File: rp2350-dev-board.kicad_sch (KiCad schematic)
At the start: 49 parts, among them J1 USB4105-GF-A, J2 Conn_02x20_Odd_Even, J3 Conn_02x20_Odd_Even, SW1 RST, SW2 BOOTSEL, U1 W25Q128JVS, U2 RP2350B, U3 TPS6285021HQDRLRQ1, U4 LM66100DCK, Y1 ABM8-272-T3 12MHz/10pF

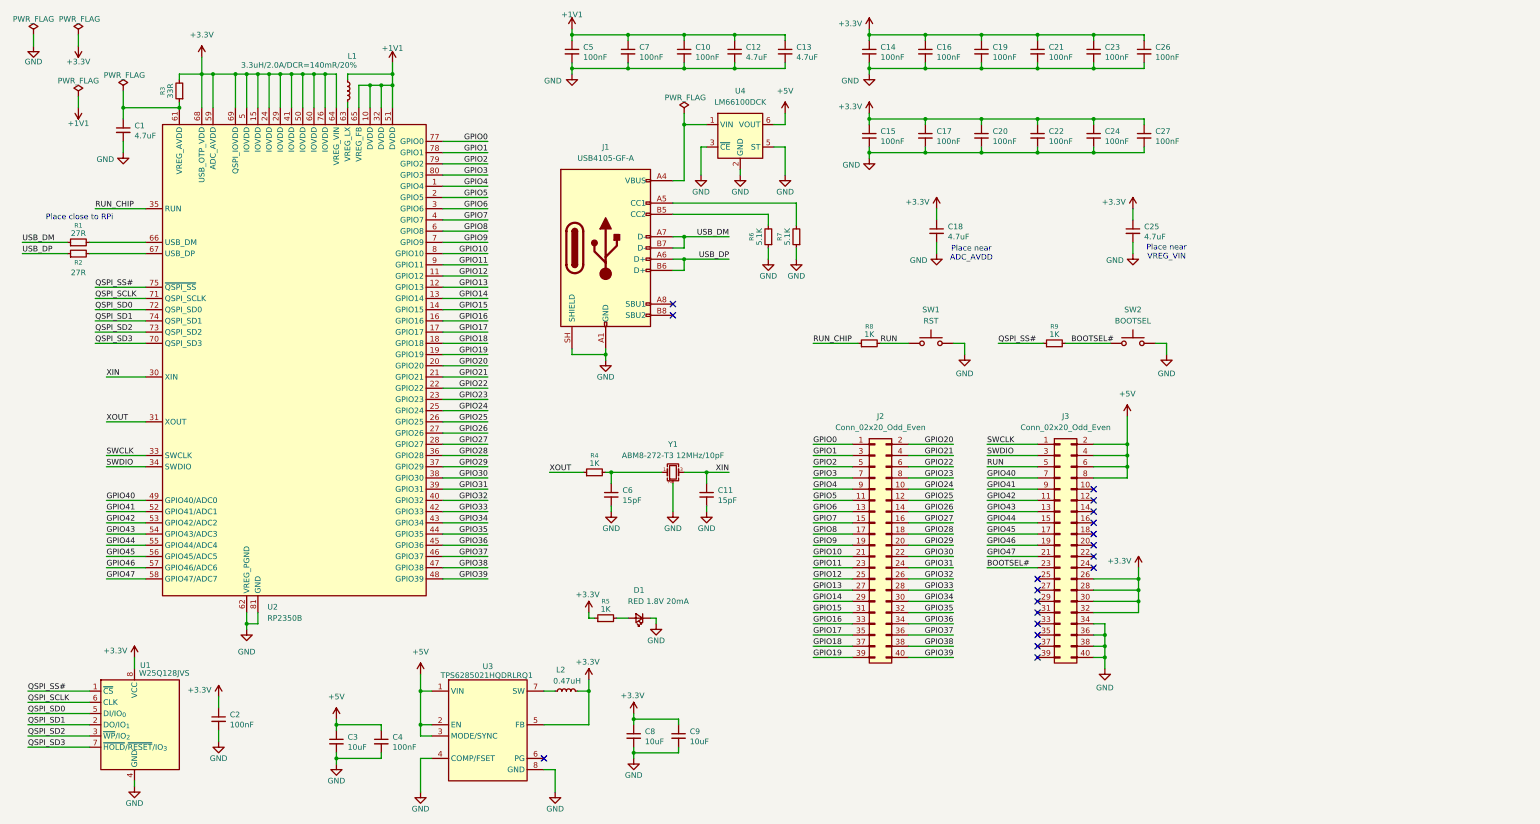
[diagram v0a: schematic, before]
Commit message: initial layout
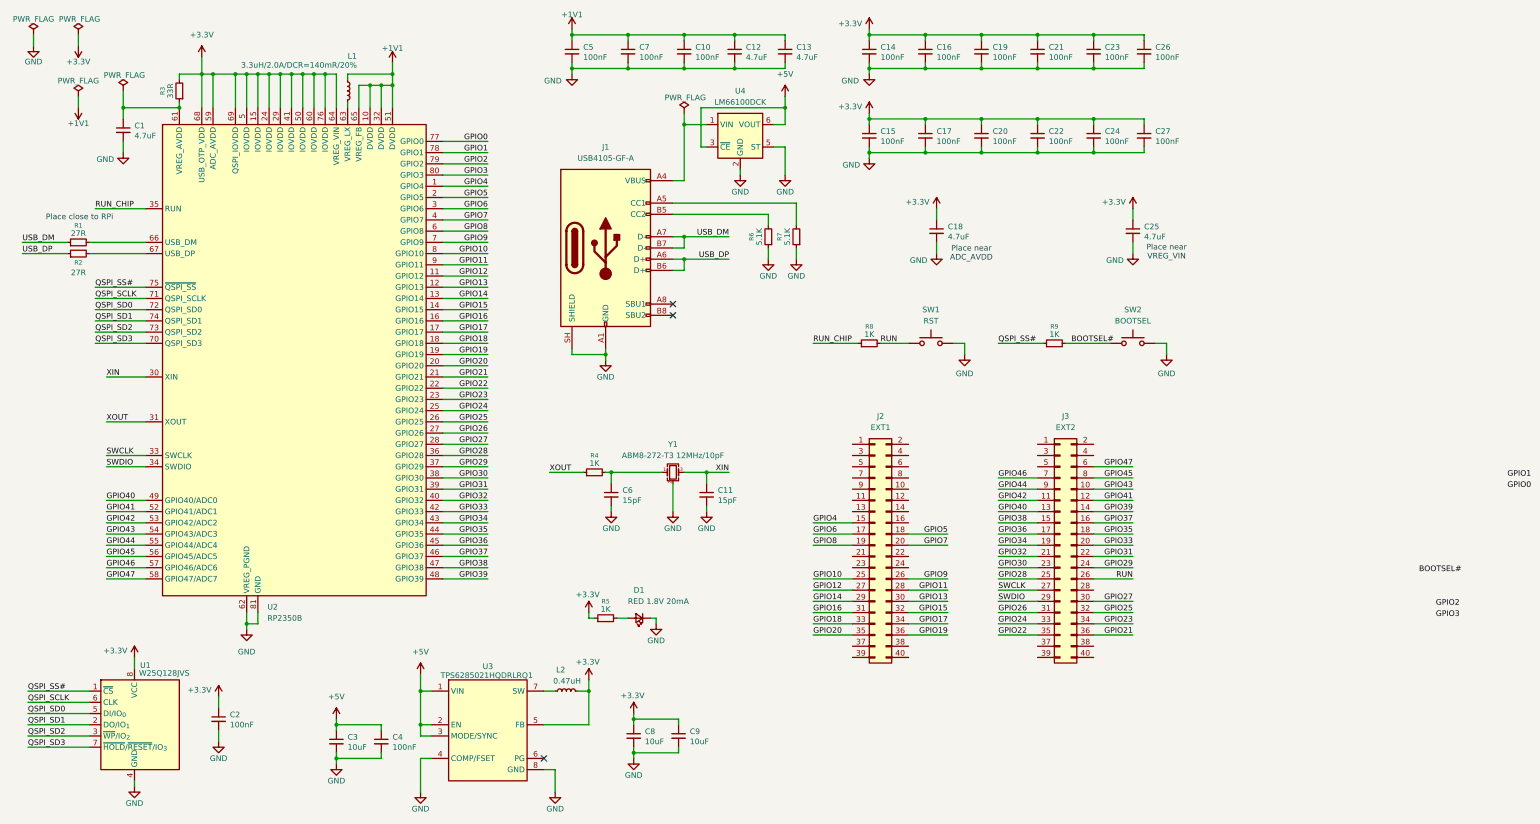
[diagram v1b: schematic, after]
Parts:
- J2: value Conn_02x20_Odd_Even -> EXT1
- J3: value Conn_02x20_Odd_Even -> EXT2
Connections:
- net +3.3V: no longer J3.26 (Pin_26), J3.28 (Pin_28), J3.30 (Pin_30), J3.32 (Pin_32)
- net +5V: now also U4.3 (~{CE}); no longer J3.2 (Pin_2), J3.4 (Pin_4), J3.6 (Pin_6), J3.8 (Pin_8)
- net BOOTSEL#: no longer J3.23 (Pin_23)
- net GND: no longer J3.34 (Pin_34), J3.36 (Pin_36), J3.38 (Pin_38), J3.40 (Pin_40), U4.3 (~{CE})
- net GPIO0: no longer J2.1 (Pin_1)
- net GPIO1: no longer J2.3 (Pin_3)
- net GPIO10: now also J2.25 (Pin_25); no longer J2.21 (Pin_21)
- net GPIO11: now also J2.28 (Pin_28); no longer J2.23 (Pin_23)
- net GPIO12: now also J2.27 (Pin_27); no longer J2.25 (Pin_25)
- net GPIO13: now also J2.30 (Pin_30); no longer J2.27 (Pin_27)
- net GPIO15: now also J2.32 (Pin_32); no longer J2.31 (Pin_31)
- net GPIO16: now also J2.31 (Pin_31); no longer J2.33 (Pin_33)
- net GPIO17: now also J2.34 (Pin_34); no longer J2.35 (Pin_35)
- net GPIO18: now also J2.33 (Pin_33); no longer J2.37 (Pin_37)
- net GPIO19: now also J2.36 (Pin_36); no longer J2.39 (Pin_39)
- net GPIO2: no longer J2.5 (Pin_5)
- net GPIO20: now also J2.35 (Pin_35); no longer J2.2 (Pin_2)
- net GPIO21: now also J3.36 (Pin_36); no longer J2.4 (Pin_4)
- net GPIO22: now also J3.35 (Pin_35); no longer J2.6 (Pin_6)
- net GPIO23: now also J3.34 (Pin_34); no longer J2.8 (Pin_8)
- net GPIO24: now also J3.33 (Pin_33); no longer J2.10 (Pin_10)
- net GPIO25: now also J3.32 (Pin_32); no longer J2.12 (Pin_12)
- net GPIO26: now also J3.31 (Pin_31); no longer J2.14 (Pin_14)
- net GPIO27: now also J3.30 (Pin_30); no longer J2.16 (Pin_16)
- net GPIO28: now also J3.25 (Pin_25); no longer J2.18 (Pin_18)
- net GPIO29: now also J3.24 (Pin_24); no longer J2.20 (Pin_20)
- net GPIO3: no longer J2.7 (Pin_7)
- net GPIO30: now also J3.23 (Pin_23); no longer J2.22 (Pin_22)
- net GPIO31: now also J3.22 (Pin_22); no longer J2.24 (Pin_24)
- net GPIO32: now also J3.21 (Pin_21); no longer J2.26 (Pin_26)
- net GPIO33: now also J3.20 (Pin_20); no longer J2.28 (Pin_28)
- net GPIO34: now also J3.19 (Pin_19); no longer J2.30 (Pin_30)
- net GPIO35: now also J3.18 (Pin_18); no longer J2.32 (Pin_32)
- net GPIO36: now also J3.17 (Pin_17); no longer J2.34 (Pin_34)
- net GPIO37: now also J3.16 (Pin_16); no longer J2.36 (Pin_36)
- net GPIO38: now also J3.15 (Pin_15); no longer J2.38 (Pin_38)
- net GPIO39: now also J3.14 (Pin_14); no longer J2.40 (Pin_40)
- net GPIO4: now also J2.15 (Pin_15); no longer J2.9 (Pin_9)
- net GPIO40: now also J3.13 (Pin_13); no longer J3.7 (Pin_7)
- net GPIO41: now also J3.12 (Pin_12); no longer J3.9 (Pin_9)
- net GPIO43: now also J3.10 (Pin_10); no longer J3.13 (Pin_13)
- net GPIO44: now also J3.9 (Pin_9); no longer J3.15 (Pin_15)
- net GPIO45: now also J3.8 (Pin_8); no longer J3.17 (Pin_17)
- net GPIO46: now also J3.7 (Pin_7); no longer J3.19 (Pin_19)
- net GPIO47: now also J3.6 (Pin_6); no longer J3.21 (Pin_21)
- net GPIO5: now also J2.18 (Pin_18); no longer J2.11 (Pin_11)
- net GPIO6: now also J2.17 (Pin_17); no longer J2.13 (Pin_13)
- net GPIO7: now also J2.20 (Pin_20); no longer J2.15 (Pin_15)
- net GPIO8: now also J2.19 (Pin_19); no longer J2.17 (Pin_17)
- net GPIO9: now also J2.26 (Pin_26); no longer J2.19 (Pin_19)
- net RUN: now also J3.26 (Pin_26); no longer J3.5 (Pin_5)
- net SWCLK: now also J3.27 (Pin_27); no longer J3.1 (Pin_1)
- net SWDIO: now also J3.29 (Pin_29); no longer J3.3 (Pin_3)
- no-connect marks 19 -> 3

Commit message: wip
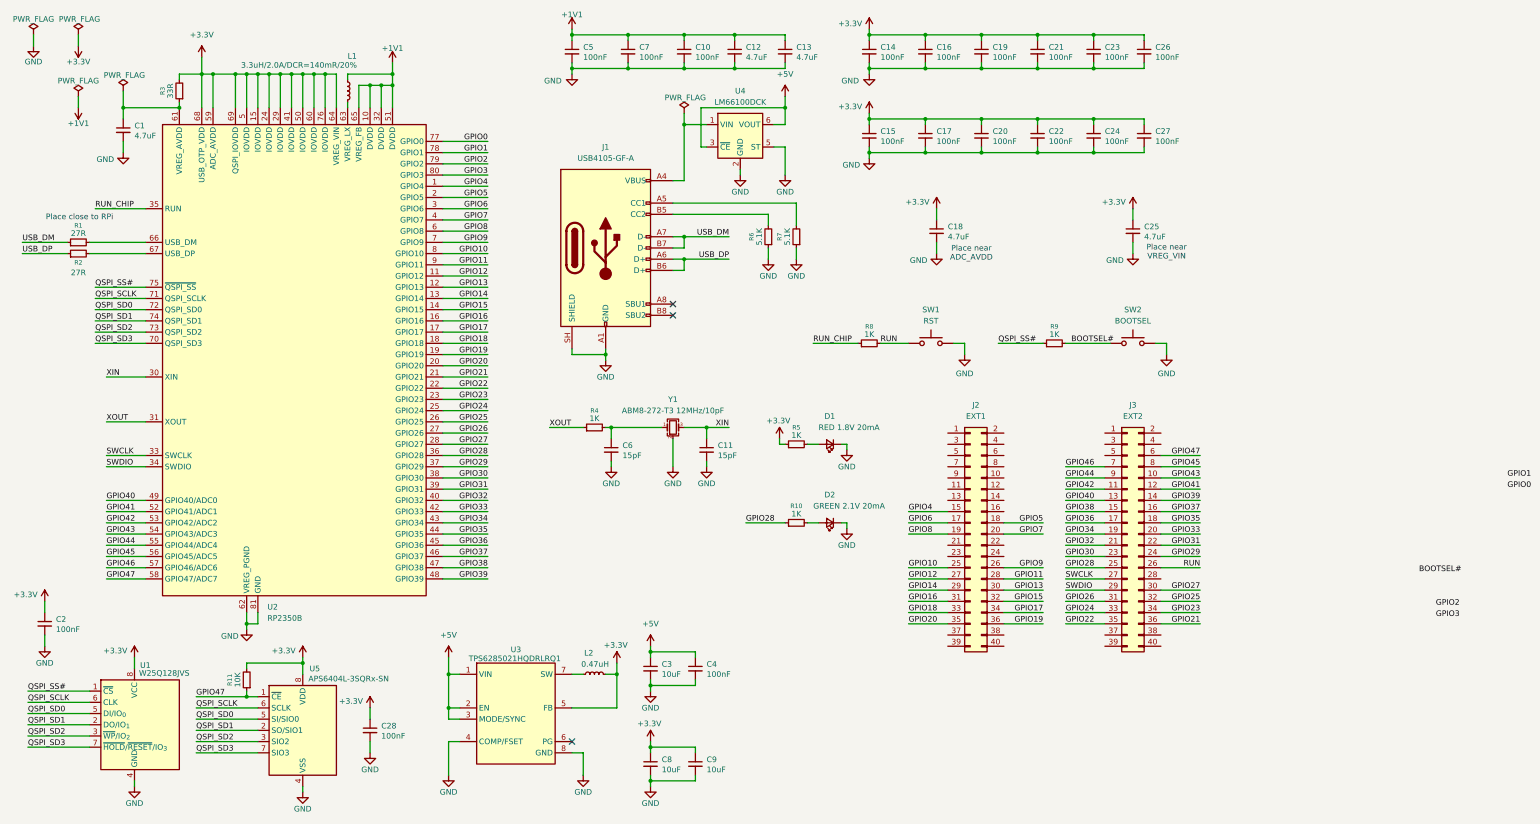
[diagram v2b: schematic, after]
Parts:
- added C28: 100nF, Capacitor_SMD:C_0402_1005Metric_Pad0.74x0.62mm_HandSolder, symbol Device:C_Small
- added D2: GREEN 2.1V 20mA, LED_SMD:LED_0805_2012Metric_Pad1.15x1.40mm_HandSolder, symbol Device:LED_Small
- added R10: 1K, Resistor_SMD:R_0805_2012Metric_Pad1.20x1.40mm_HandSolder, symbol Device:R_Small
- added R11: 10K, Resistor_SMD:R_0805_2012Metric_Pad1.20x1.40mm_HandSolder, symbol Device:R_Small
- added U5: APS6404L-3SQRx-SN, Package_SO:SOIC-8_3.9x4.9mm_P1.27mm, symbol Memory_RAM:APS6404L-3SQRx-SN
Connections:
- net +3.3V: now also C28.1, R11.2, U5.8 (VDD)
- net GND: now also C28.2, D2.1 (K), U5.4 (VSS)
- net GPIO28: now also R10.1
- net GPIO47: now also R11.1, U5.1 (~{CE})
- net QSPI_SCLK: now also U5.6 (SCLK)
- net QSPI_SD0: now also U5.5 (SI/SIO0)
- net QSPI_SD1: now also U5.2 (SO/SIO1)
- net QSPI_SD2: now also U5.3 (SIO2)
- net QSPI_SD3: now also U5.7 (SIO3)
- new net: D2.2 (A), R10.2
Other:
- moved on the sheet: C11, C2, C3, C4, C6, C8, C9, D1, J2, J3, L2, R4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
